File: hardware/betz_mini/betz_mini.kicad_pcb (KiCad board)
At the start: 4 copper layers, 35 x 35 mm, 35 parts, among them J1 upstream, J2 downstream, J3 ARM SWD, J4 BLDC, J5 BONUS, U1 stm32g474ceu6, U2 AS5047U, U3 IIS328DQ, U4 MP6540, U5 LMZM23601V3, U6 THVD2450, X1 8 MHz

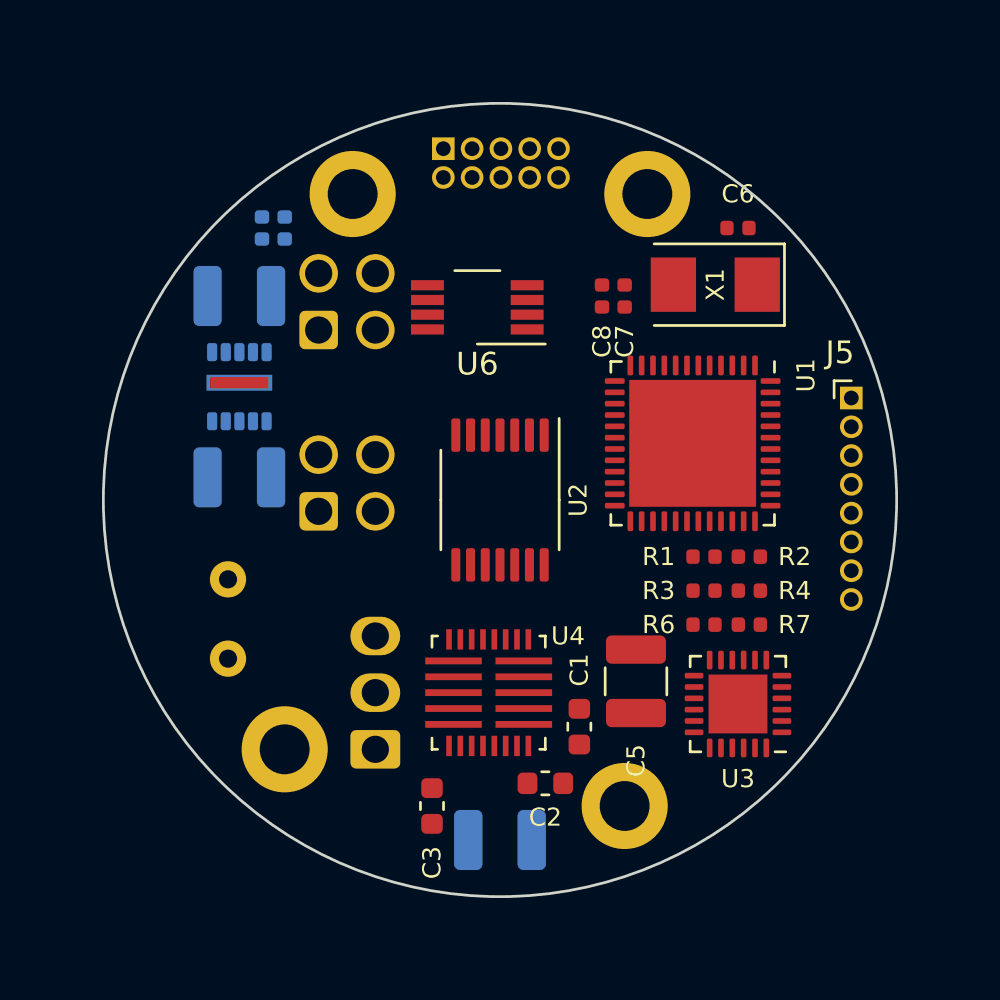
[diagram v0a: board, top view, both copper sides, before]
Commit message: WIP betz mini
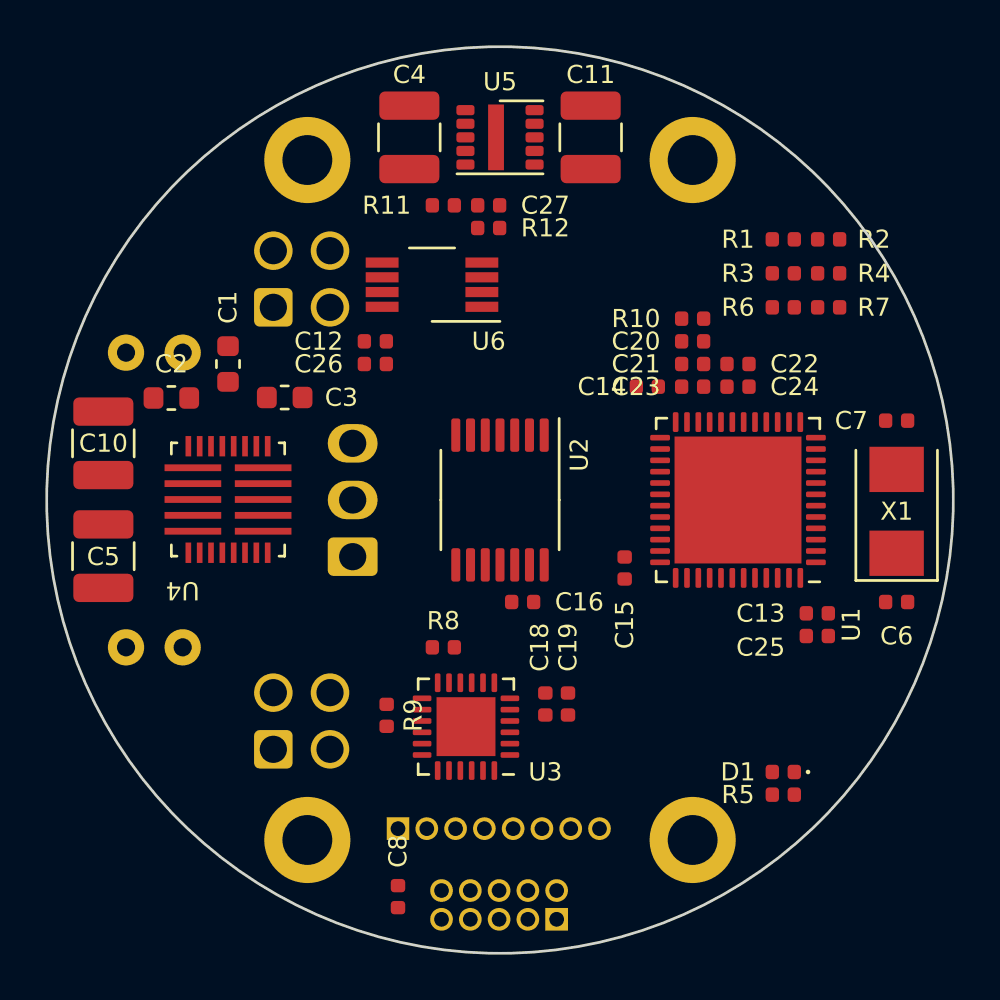
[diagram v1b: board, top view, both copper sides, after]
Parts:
- added C12: 100n, Capacitor_SMD:C_0402_1005Metric, F.Cu at (144.5, 93.0)
- added C13: 100n, Capacitor_SMD:C_0402_1005Metric, F.Cu at (164.0, 105.0)
- added C14: 100n, Capacitor_SMD:C_0402_1005Metric, F.Cu at (156.5, 95.0)
- added C15: 100n, Capacitor_SMD:C_0402_1005Metric, F.Cu at (155.5, 103.0)
- added C16: 100n, Capacitor_SMD:C_0402_1005Metric, F.Cu at (151.0, 104.5)
- added C17: 100u, Capacitor_THT:C_Radial_D6.3mm_H11.0mm_P2.50mm, B.Cu at (133.5, 93.5)
- added C18: 100n, Capacitor_SMD:C_0402_1005Metric, F.Cu at (152.0, 109.0)
- added C19: 1u, Capacitor_SMD:C_0402_1005Metric, F.Cu at (153.0, 109.0)
- added C20: 10u, Capacitor_SMD:C_0402_1005Metric, F.Cu at (158.5, 93.0)
- added C21: 1u, Capacitor_SMD:C_0402_1005Metric, F.Cu at (158.5, 94.0)
- added C22: 1u, Capacitor_SMD:C_0402_1005Metric, F.Cu at (160.5, 94.0)
- added C23: 100n, Capacitor_SMD:C_0402_1005Metric, F.Cu at (158.5, 95.0)
- added C24: 100n, Capacitor_SMD:C_0402_1005Metric, F.Cu at (160.5, 95.0)
- added C25: 10u, Capacitor_SMD:C_0402_1005Metric, F.Cu at (164.0, 106.0)
- added C26: 1u, Capacitor_SMD:C_0402_1005Metric, F.Cu at (144.5, 94.0)
- added C27: 100n, Capacitor_SMD:C_0402_1005Metric, F.Cu at (149.5, 87.0)
- added R10: ferrite, Resistor_SMD:R_0402_1005Metric, F.Cu at (158.5, 92.0)
- added R11: 100k, Resistor_SMD:R_0402_1005Metric, F.Cu at (147.5, 87.0)
- added R12: 4k7, Resistor_SMD:R_0402_1005Metric, F.Cu at (149.5, 88.0)
- added R8: 4k7, Resistor_SMD:R_0402_1005Metric, F.Cu at (147.5, 106.5)
- added R9: 4k7, Resistor_SMD:R_0402_1005Metric, F.Cu at (145.0, 109.5)
- C10, C11, C4, D1, R5, U5: moved to F.Cu
- C9: value 470u -> 100u; footprint Capacitor_THT:C_Radial_D8.0mm_H11.5mm_P3.50mm -> Capacitor_THT:C_Radial_D6.3mm_H11.0mm_P2.50mm
- J5: footprint Connector_PinHeader_1.27mm:PinHeader_1x08_P1.27mm_Horizontal -> Connector_PinHeader_1.27mm:PinHeader_1x08_P1.27mm_Vertical; moved to B.Cu
- moved J3 34.4 mm to (152.5, 118.5), turned to 90 degrees
- moved R5 34.0 mm to (162.5, 113.0), turned to 0 degrees
- moved D1 32.6 mm to (162.5, 112.0), turned to 180 degrees
- moved C8 28.0 mm to (145.5, 117.5), turned to -90 degrees
- moved J5 27.6 mm to (145.5, 114.5), turned to -90 degrees
- moved C10 24.7 mm to (132.5, 97.5), turned to 90 degrees
- moved C5 24.1 mm to (132.5, 102.5), turned to -90 degrees
- moved C2 23.7 mm to (135.5, 95.5), turned to 180 degrees
- moved C1 22.3 mm to (138.0, 94.0)
- moved C11 21.6 mm to (154.0, 84.0), turned to 90 degrees
- moved C3 19.2 mm to (140.5, 95.5), turned to 0 degrees
- moved C6 17.9 mm to (167.5, 104.5), turned to 0 degrees
- moved U5 15.9 mm to (150.0, 84.0), turned to 0 degrees
- moved R1 14.4 mm to (162.5, 88.5)
- moved R2 14.4 mm to (164.5, 88.5)
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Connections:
- J5 pad 1: /DEBUG_TX -> GND
- J5 pad 2: Net-(J5-Pad2) -> +3V3
- J5 pad 3: Net-(J5-Pad3) -> /DEBUG_TX
- J5 pad 4: Net-(J5-Pad4) -> /BONUS_MOSI
- J5 pad 5: Net-(J5-Pad5) -> /BONUS_MISO
- J5 pad 6: Net-(J5-Pad6) -> /BONUS_SCK
- J5 pad 7: Net-(J5-Pad7) -> /BONUS_GPIO
- J5 pad 8: GND -> /BONUS_CS
- U1 pad 10: Net-(U1-Pad10) -> /RS485_DI
- U1 pad 11: Net-(U1-Pad11) -> /RS485_RO
- U1 pad 15: Net-(U1-Pad15) -> /IB
- U1 pad 18: Net-(U1-Pad18) -> /IA
- U1 pad 24: Net-(U1-Pad24) -> /ENC_CS
- U1 pad 25: Net-(U1-Pad25) -> /VBUS_DIV
- U1 pad 26: Net-(U1-Pad26) -> /ENC_SCK
- U1 pad 27: Net-(U1-Pad27) -> /ENC_MISO
- U1 pad 28: Net-(U1-Pad28) -> /ENC_MOSI
- U1 pad 29: Net-(U1-Pad29) -> /BLDC_EN
- U1 pad 30: Net-(U1-Pad30) -> /PWMC
- U1 pad 31: Net-(U1-Pad31) -> /PWMB
- U1 pad 32: Net-(U1-Pad32) -> /PWMA
- U1 pad 33: Net-(U1-Pad33) -> /SLEEP
- U1 pad 34: Net-(U1-Pad34) -> /FAULT
- U1 pad 38: Net-(U1-Pad38) -> /ACCEL_SCL
- U1 pad 39: Net-(U1-Pad39) -> /BONUS_SCK
- U1 pad 40: Net-(U1-Pad40) -> /BONUS_MISO
- U1 pad 41: Net-(U1-Pad41) -> /BONUS_GPIO
- U1 pad 42: Net-(U1-Pad42) -> /BONUS_CS
- U1 pad 43: Net-(U1-Pad43) -> /BONUS_MOSI
- U1 pad 44: Net-(U1-Pad44) -> /DEBUG_TX
- U1 pad 45: Net-(U1-Pad45) -> /ACCEL_SDA
- U1 pad 46: Net-(U1-Pad46) -> GND
- U1 pad 47: Net-(U1-Pad47) -> /STATUS_LED
- U1 pad 49: Net-(U1-Pad49) -> GND
- U1 pad 8: Net-(U1-Pad8) -> /IC
- U1 pad 9: Net-(U1-Pad9) -> /RS485_DE
- U2 pad 1: Net-(U2-Pad1) -> /ENC_CS
- U2 pad 11: Net-(U2-Pad11) -> +3V3
- U2 pad 12: Net-(U2-Pad12) -> +3V3
- U2 pad 13: Net-(U2-Pad13) -> GND
- U2 pad 2: Net-(U2-Pad2) -> /ENC_SCK
- U2 pad 3: Net-(U2-Pad3) -> /ENC_MISO
- U2 pad 4: Net-(U2-Pad4) -> /ENC_MOSI
- U2 pad 5: Net-(U2-Pad5) -> GND
- U3 pad 10: Net-(U3-Pad10) -> GND
- U3 pad 11: Net-(U3-Pad11) -> /ACCEL_SCL
- U3 pad 12: Net-(U3-Pad12) -> +3V3
- U3 pad 13: Net-(U3-Pad13) -> +3V3
- U3 pad 14: Net-(U3-Pad14) -> +3V3
- U3 pad 15: Net-(U3-Pad15) -> GND
- U3 pad 16: Net-(U3-Pad16) -> /ACCEL_SDA
- U3 pad 25: Net-(U3-Pad25) -> GND
- U3 pad 4: Net-(U3-Pad4) -> GND
- U3 pad 5: Net-(U3-Pad5) -> +3V3
- U3 pad 6: Net-(U3-Pad6) -> GND
- U3 pad 8: Net-(U3-Pad8) -> GND
- U3 pad 9: Net-(U3-Pad9) -> GND
- U4 pad 3: /ENA -> /BLDC_EN
- U4 pad 4: /ENB -> /BLDC_EN
- U4 pad 5: /ENC -> /BLDC_EN
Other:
- board size 35 x 35 mm -> 40 x 40 mm
